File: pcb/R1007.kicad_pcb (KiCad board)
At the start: 4 copper layers, 69 x 44 mm, 41 parts, among them J1 CONN500P-01X08, J2 CONN500P-01X04, J3 CONN_R1000A_EXTENSION, Q1 PSMN1R2-30YLC, Q2 PSMN1R2-30YLC, Q3 PSMN1R2-30YLC, Q4 PSMN1R2-30YLC, U1 74HC125, U2 AS78L05ZTR-E1, U3 TLP293-4

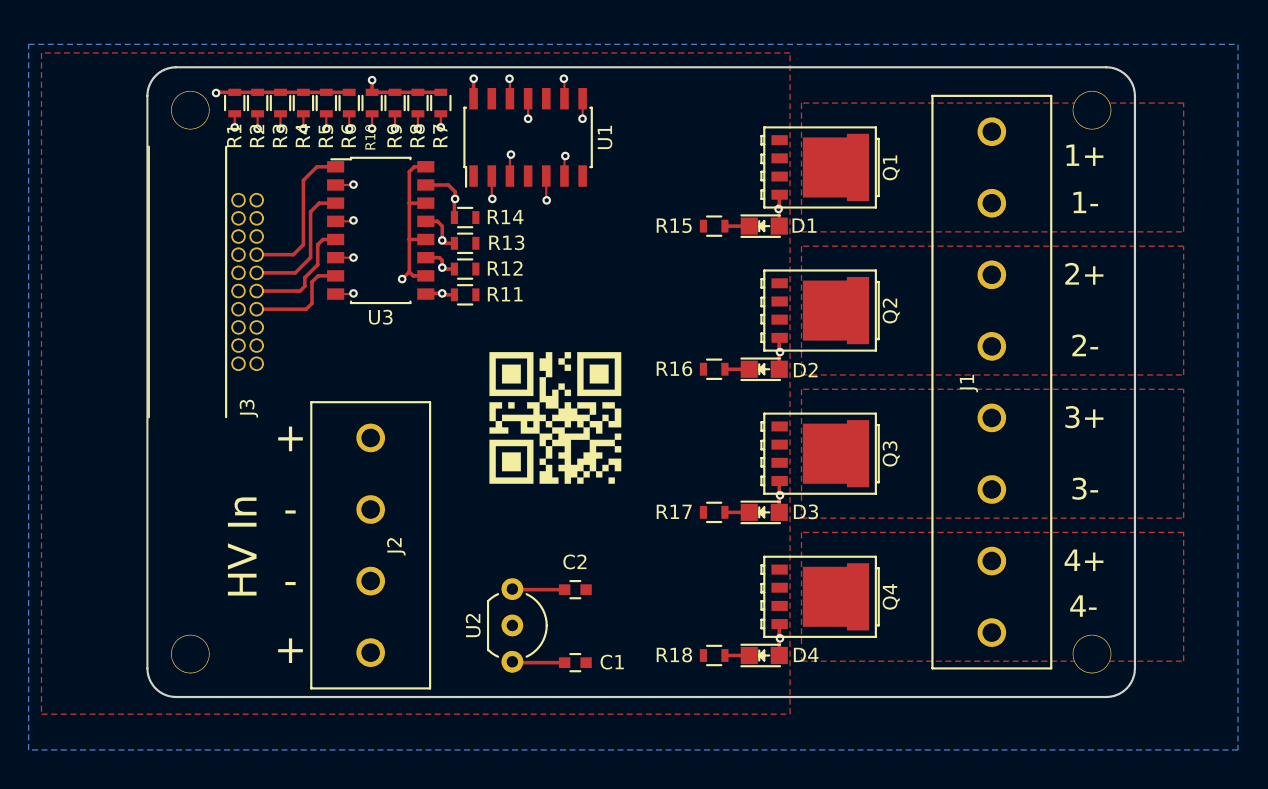
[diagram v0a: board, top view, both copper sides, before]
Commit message: completed layout, wip
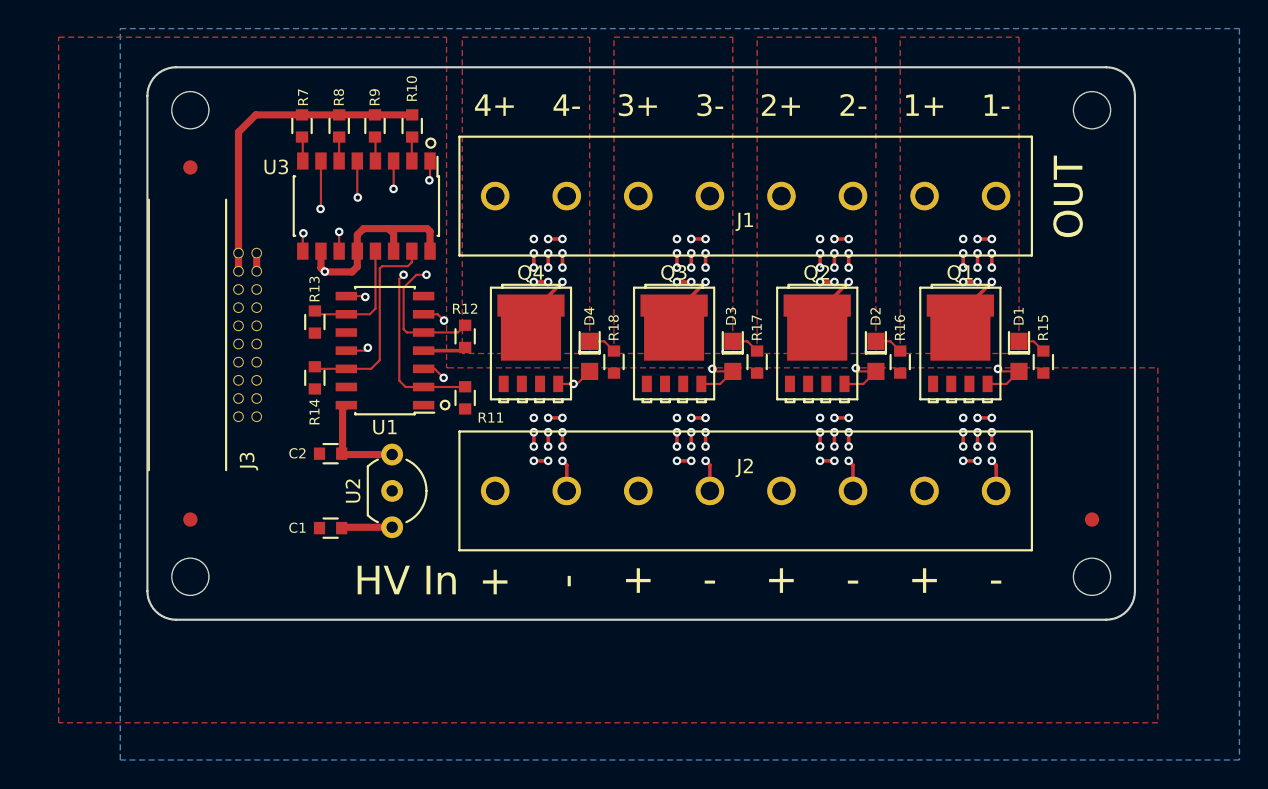
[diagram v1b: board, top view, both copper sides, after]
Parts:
- removed G***: LOGO, pluggee:pluggee-QRNEG-127X127
- removed G***: LOGO, pluggee:pluggee-LOGO-131X127
- removed G***: LOGO, pluggee:pluggee-QRNEG-190X190
- removed R1, R2, R3, R4, R5, R6: 10k, Resistors_SMD:R_0603
- added A1: ART, pluggee:pluggeeLabsIcon-13X7, B.Cu at (159.4, 87.0)
- added FID1: FIDTOP001, Main:FIDTOP001, F.Cu at (106.0, 99.6)
- added FID2: FIDTOP001, Main:FIDTOP001, F.Cu at (169.0, 99.6)
- added FID3: FIDTOP001, Main:FIDTOP001, F.Cu at (106.0, 75.0)
- C1, C2: value 1uF -> CC0603KRX7R9BB104; footprint Capacitors_SMD:C_0603 -> Main:CAPC0603
- D1, D2, D3, D4: value Led_Small -> LTW-170TK; footprint LEDs:LED_0805 -> Main:DIOC200X120X110
- J2: value CONN500P-01X04 -> CONN500P-01X08; footprint Main:CONN500P-01X04 -> Main:CONN500P-01X08
- R10, R15, R16, R17, R18, R7, R8, R9: value 1k -> RC0603FR-071KL; footprint Resistors_SMD:R_0603 -> Main:RESC0603
- R11, R12, R13, R14: value 4.7k -> RC0603FR-074K7L; footprint Resistors_SMD:R_0603 -> Main:RESC0603
- moved Q4 26.9 mm to (129.8, 87.3), turned to 0 degrees
- moved J2 26.5 mm to (144.8, 97.6), turned to 0 degrees
- moved R15 24.9 mm to (165.6, 88.6), turned to 270 degrees
- moved D4 24.2 mm to (133.9, 88.2), turned to 270 degrees
- moved R18 21.7 mm to (135.6, 88.6), turned to 270 degrees
- moved J1 21.6 mm to (144.8, 77.0), turned to 180 degrees
- moved D1 20.0 mm to (163.9, 88.2), turned to 270 degrees
- moved C2 19.6 mm to (115.8, 95.0), turned to 180 degrees
- moved C1 19.5 mm to (115.8, 100.2), turned to 180 degrees
- moved U1 17.9 mm to (119.6, 87.8), turned to 180 degrees
- moved Q1 15.7 mm to (159.8, 87.3), turned to 0 degrees
- moved R14 15.4 mm to (114.7, 89.7), turned to 270 degrees
- moved R16 13.0 mm to (155.6, 88.6), turned to 270 degrees
- moved Q3 12.8 mm to (139.8, 87.3), turned to 0 degrees
- moved U2 12.6 mm to (120.1, 97.6)
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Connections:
- J1 pad 1: /N4 -> /N1
- J1 pad 3: /N3 -> /N2
- J1 pad 5: /N2 -> /N3
- J1 pad 7: /N1 -> /N4
- J2 pad 3: GNDPWR -> VDD
- J2 pad 4: VDD -> GNDPWR
- J3 pad 1: ~MRESET -> (no net)
- J3 pad 10: ID2 -> (no net)
- J3 pad 12: ID1 -> (no net)
- J3 pad 14: ID0 -> (no net)
- J3 pad 16: +3V3 -> (no net)
- J3 pad 2: C2D -> (no net)
- J3 pad 8: ID3 -> (no net)
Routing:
- net GNDPWR: track 0.00 -> 55.9 mm, vias 0 -> 48
- net /GN4: track 52.9 -> 13.5 mm
- net ~MRESET: track 36.9 -> 0.00 mm, vias 1 -> 0
- net /GN1: track 31.0 -> 58.5 mm
- net C2D: track 23.8 -> 0.00 mm, vias 1 -> 0
- net +5P: track 17.7 -> 39.6 mm, vias 2 -> 1
- net +3V3: track 21.3 -> 0.00 mm, vias 1 -> 0
- net ID3: track 21.1 -> 0.00 mm, vias 1 -> 0
- net ID2: track 20.6 -> 0.00 mm, vias 1 -> 0
- net ID1: track 19.6 -> 0.00 mm, vias 1 -> 0
- net ID0: track 18.9 -> 0.00 mm, vias 1 -> 0
- net /INR4: track 17.9 -> 1.70 mm, vias 2 -> 0
- net /N2: track 0.00 -> 15.8 mm, vias 0 -> 12
- net /N1: track 0.00 -> 15.8 mm, vias 0 -> 12
- net /N4: track 2.20 -> 14.9 mm, vias 0 -> 12
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- added copper zone on In1.Cu, net /N1
- added copper zone on In1.Cu, net /N2
- added copper zone on In1.Cu, net /N3
- added copper zone on In1.Cu, net /N4
- added copper zone on In1.Cu, net GNDPWR
- removed copper zone on In1.Cu, net +5P
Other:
- board size 69 x 44 mm -> 69 x 38.6 mm
- board text added: "OUT"
- board text added: "R1007 v1.1 Quad 20A NFET Drivers plugg.ee Labs LLC http://plugg.ee"
- board text removed: "R1007 v1.0.0 Quad 20A NFET Drivers plugg.ee Labs 2016 http://plugg.ee"
